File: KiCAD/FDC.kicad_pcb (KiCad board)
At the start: 2 copper layers, 53.5 x 110.5 mm, 21 parts, among them J1 Other Signals, Q1 FDV301N, Q2 FDV301N, U1 74HCT245, U2 74HCT245, U3 74HCT245, U6 Z80, U7 Z80

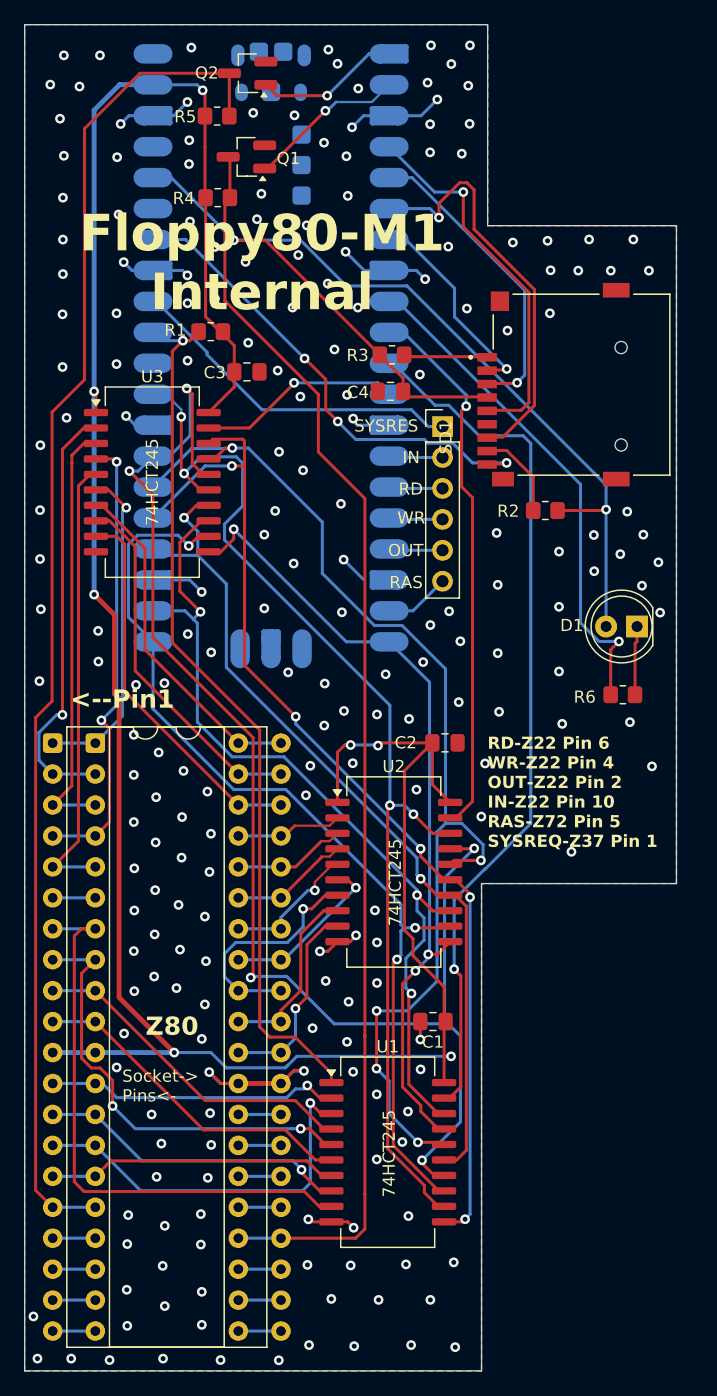
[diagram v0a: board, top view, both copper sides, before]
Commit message: New board revision
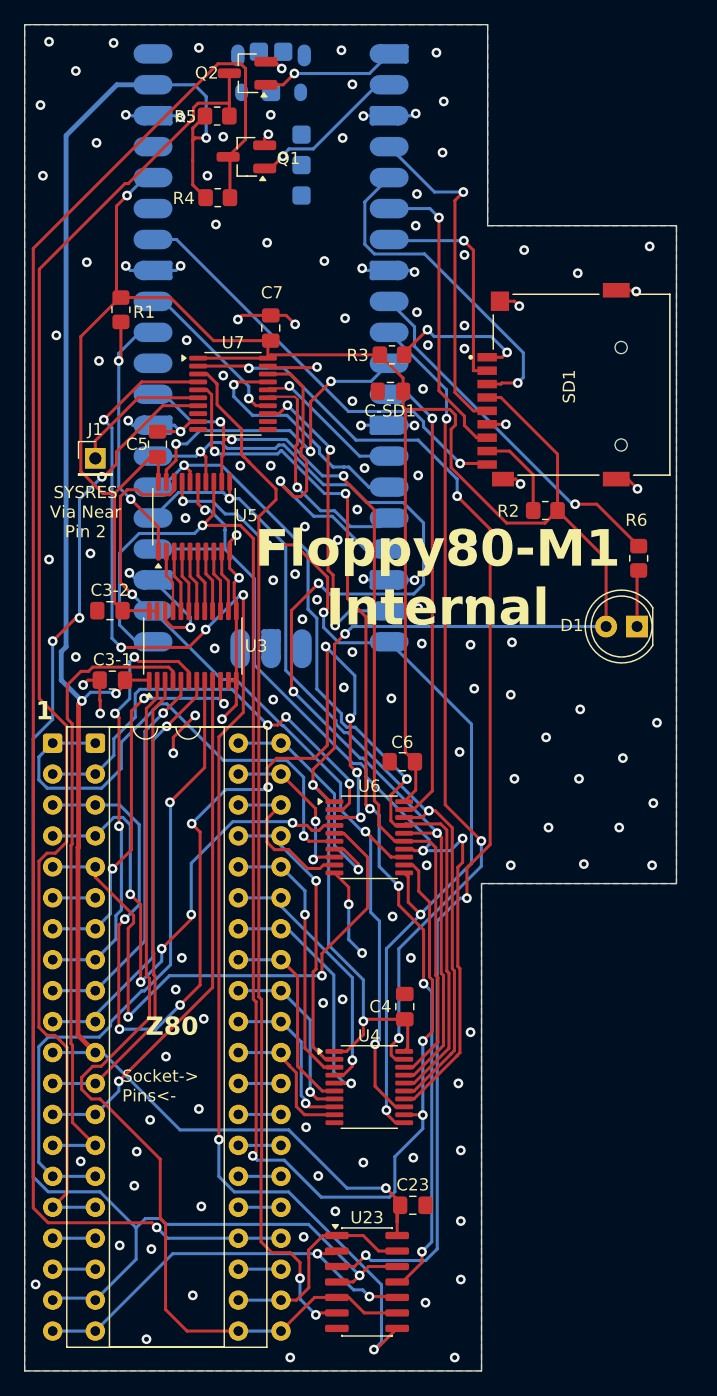
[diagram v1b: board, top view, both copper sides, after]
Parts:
- removed C1, C2, C3: 100nF, Capacitor_SMD:C_0805_2012Metric_Pad1.18x1.45mm_HandSolder
- removed the U1 at (156.3, 131.1)
- removed the U2 at (156.8, 108.0)
- added C23: 100nF, Capacitor_SMD:C_0805_2012Metric_Pad1.18x1.45mm_HandSolder, F.Cu at (158.4, 135.4)
- added C3-1: 100nF, Capacitor_SMD:C_0805_2012Metric_Pad1.18x1.45mm_HandSolder, F.Cu at (133.7, 92.3)
- added C3-2: 100nF, Capacitor_SMD:C_0805_2012Metric_Pad1.18x1.45mm_HandSolder, F.Cu at (133.5, 86.6)
- added C4: 100nF, Capacitor_SMD:C_0805_2012Metric_Pad1.18x1.45mm_HandSolder, F.Cu at (157.7, 119.1)
- added C5: 100nF, Capacitor_SMD:C_0805_2012Metric_Pad1.18x1.45mm_HandSolder, F.Cu at (137.4, 72.9)
- added C6: 100nF, Capacitor_SMD:C_0805_2012Metric_Pad1.18x1.45mm_HandSolder, F.Cu at (157.5, 99.0)
- added C7: 100nF, Capacitor_SMD:C_0805_2012Metric_Pad1.18x1.45mm_HandSolder, F.Cu at (146.7, 63.4)
- added U23: SN74LS32NSR, Package_SO:SOIC-14_3.9x8.7mm_P1.27mm, F.Cu at (154.6, 141.7)
- added U4: SN74LVC245APWR, Package_SO:TSSOP-20_4.4x6.5mm_P0.65mm, F.Cu at (154.8, 125.7)
- added U5: SN74LVC245APWR, Package_SO:TSSOP-20_4.4x6.5mm_P0.65mm, F.Cu at (140.4, 78.9)
- added U6: SN74LVC245APWR, Package_SO:TSSOP-20_4.4x6.5mm_P0.65mm, F.Cu at (154.8, 105.2)
- added U7: SN74LVC245APWR, Package_SO:TSSOP-20_4.4x6.5mm_P0.65mm, F.Cu at (143.6, 68.8)
- J1: value Other Signals -> Conn_01x01_Pin; footprint Connector_PinHeader_2.54mm:PinHeader_1x06_P2.54mm_Vertical -> Connector_PinHeader_2.54mm:PinHeader_1x01_P2.54mm_Vertical
- U3: value 74HCT245 -> SN74LVCC4245APWR; footprint Package_SO:SOIC-20W_7.5x15.4mm_P1.27mm -> Package_SO:TSSOP-24_4.4x7.8mm_P0.65mm
- moved J1 28.6 mm to (132.3, 74.1)
- moved U3 13.9 mm to (140.3, 89.5), turned to 90 degrees
- moved R6 11.3 mm to (176.9, 82.3), turned to 90 degrees
- moved R1 7.59 mm to (134.4, 61.9), turned to 90 degrees
- renumbered C4 to C-SD1, U7 to U1, U6 to U2
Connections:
- J1 pad 1: /SYSRES' -> /SYSRES*
- R1 pad 2: +5V -> +3V3
- U3 pad 10: GND -> /D4
- U3 pad 11: /D0' -> GND
- U3 pad 12: /D1' -> GND
- U3 pad 13: /D2' -> GND
- U3 pad 14: /D3' -> /D4-
- U3 pad 15: /D7' -> /D7-
- U3 pad 16: /D6' -> /D1-
- U3 pad 17: /D5' -> /D6-
- U3 pad 18: /D4' -> /D3-
- U3 pad 19: /ADDRH_OE -> /D5-
- U3 pad 2: /A12 -> /RD*
- U3 pad 20: +5V -> /D0-
- U3 pad 3: /A13 -> /D2
- U3 pad 4: /A14 -> /D0
- U3 pad 5: /A15 -> /D5
- U3 pad 6: /A11 -> /D3
- U3 pad 7: /A10 -> /D6
- U3 pad 8: /A9 -> /D1
- U3 pad 9: /A8 -> /D7
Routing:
- net +3V3: track 89.9 -> 231.4 mm, vias 2 -> 4
- net /MREQ: track 3.50 -> 118.4 mm, vias 0 -> 4
- net /IN5V: track 0.00 -> 114.0 mm, vias 0 -> 6
- net /OUT5V: track 0.00 -> 100.7 mm, vias 0 -> 4
- net /WR5V: track 0.00 -> 87.9 mm, vias 0 -> 6
- net /RD5V: track 0.00 -> 85.8 mm, vias 0 -> 2
- net /RD*: track 3.50 -> 79.5 mm
- net +5V: track 204.4 -> 147.5 mm, vias 7 -> 4
- net /A13: track 35.7 -> 87.6 mm, vias 0 -> 9
- net /DIR: track 72.2 -> 24.7 mm, vias 1 -> 2
- net /DATAB_OE: track 71.8 -> 27.5 mm, vias 1 -> 3
- net /D1': track 78.7 -> 120.7 mm, vias 3 -> 4
- net GND: track 62.6 -> 102.3 mm, vias 219 -> 147
- net /WAIT*: track 103.8 -> 135.2 mm, vias 0 -> 1
- net /IORQ: track 3.50 -> 34.1 mm, vias 0 -> 2
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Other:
- board text added: "1"
- board text added: "All Caps - 100NF R1,R2,R3,R4,R5 - 1k R6 - 100 OHM U3 - SN74LVCC4245APWR U4,U5,U6, U7 - SN74LVC245APWR U23 - SN74LS32NSR SD - MSD-1-A Q1,Q2 - FDV301N"
- board text added: "Floppy80-M1 ver 1.21 Internal version by dabone (2026) https://github.com/dabonetn/Floppy80-M1-Internal Original By MichaelM4 https://github.com/MichaelM4/Floppy80-M1"
- board text added: "SYSRES Via Near Pin 2"
- board text removed: "74HCT245"
- board text removed: "<--Pin1"
- board text removed: "Floppy80-M1 ver 1.01 Internal version by dabone (2026) https://github.com/dabonetn/Floppy80-M1-Internal Original By MichaelM4 https://github.com/MichaelM4/Floppy80-M1"
- board text removed: "IN"
- board text removed: "OUT"
- board text removed: "Q1,Q2 - FDV301N R1,R2,R3,R4,R5 - 1k C1,C2,C3,C4 - 100NF R6 - 100 OHM U1,U2,U3 - 74HCT245"
- board text removed: "RAS"
- board text removed: "RD"
- board text removed: "RD-Z22 Pin 6 WR-Z22 Pin 4 OUT-Z22 Pin 2 IN-Z22 Pin 10 RAS-Z72 Pin 5 SYSREQ-Z37 Pin 1"
- board text removed: "SYSRES"
- board text removed: "WR"
